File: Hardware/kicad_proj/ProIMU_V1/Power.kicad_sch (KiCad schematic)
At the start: 15 parts, among them IC1 MP2731GQC-0000-Z, SW1 SW_SPDT, U7 TPS54308, U8 TPS54308

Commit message: Updated Schematic and Layout
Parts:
- added C23, C25, C26, C28: 1uF, Capacitor_SMD:C_0402_1005Metric_Pad0.74x0.62mm_HandSolder, symbol Device:C_Small
- added C24, C27: 10uF, Capacitor_SMD:C_0402_1005Metric_Pad0.74x0.62mm_HandSolder, symbol Device:C_Small
- added D2: LED, LED_SMD:LED_0603_1608Metric, symbol Device:LED
- added L3: 1.0uH, Inductor_SMD:L_0805_2012Metric_Pad1.05x1.20mm_HandSolder, symbol Device:L
- added Q1: 2SC4213, Package_TO_SOT_SMD:SOT-323_SC-70, symbol Transistor_BJT:2SC4213
- added R14, R17, R19: 10K, Resistor_SMD:R_0402_1005Metric_Pad0.72x0.64mm_HandSolder, symbol Device:R_Small
- added R15, R16, R18: 1K, Resistor_SMD:R_0402_1005Metric_Pad0.72x0.64mm_HandSolder, symbol Device:R_Small
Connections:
- net +BATT is gone; now on net BATT: BAT1.1 (Pin_1)
- net GND: now also IC1.14 (PGND_4), IC1.15 (AGND), C23.2, C24.2, C25.2, C26.2, C27.2, Q1.2 (E), R14.1; no longer BAT1.2 (Pin_2)
- net DP: now reaches IC1.1 (DP_1)
- net DP: now also IC1.26 (DP_2), IC1.27 (DP_3)
- net INT: now reaches IC1.10 (INT)
- net NTC: now reaches IC1.11 (NTC)
- net NTC: now also R15.2, R18.1
- net VNTC: now reaches IC1.12 (VNTC)
- net VNTC: now also R18.2
- net VREF: now reaches IC1.13 (VREF)
- net VREF: now also C24.1, R17.2, R19.2
- net SYS: now reaches IC1.16 (SYS)
- net SYS: now also C25.1, L3.1
- net BATT: now reaches IC1.17 (BATT)
- net BATT: now also C26.1
- net nCE: now reaches IC1.18 (~{CE})
- net SDA: now reaches IC1.21 (SDA)
- net DISC: now reaches IC1.22 (DISC)
- net DISC: now also Q1.3 (C), R19.1
- net ILIM: now reaches IC1.24 (ILIM)
- net ILIM: now also R14.2
- net DM: now reaches IC1.25 (DM)
- net PMID: now reaches IC1.3 (PMID)
- net PMID: now also C27.1
- net SW: now reaches IC1.4 (SW)
- net SW: now also C28.2, L3.2
- net BST: now reaches IC1.8 (BST)
- net BST: now also C28.1
- net STAT: now reaches IC1.9 (STAT)
- net STAT: now also D2.1 (K)
- net BAT_I2C_SCL renamed SCL
- net BAT_OTG renamed OTG
- net USB_PWR_IN renamed IN
- net IN: now also C23.1
- new net: Q1.1 (B), R16.2
- new net: BAT1.2 (Pin_2), R15.1
- new net: D2.2 (A), R17.1
- new net DISC_PIN: R16.1
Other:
- moved on the sheet: BAT1, C12, C13, C14, C15, IC1, L1, L2, R10, R7, R8, R9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

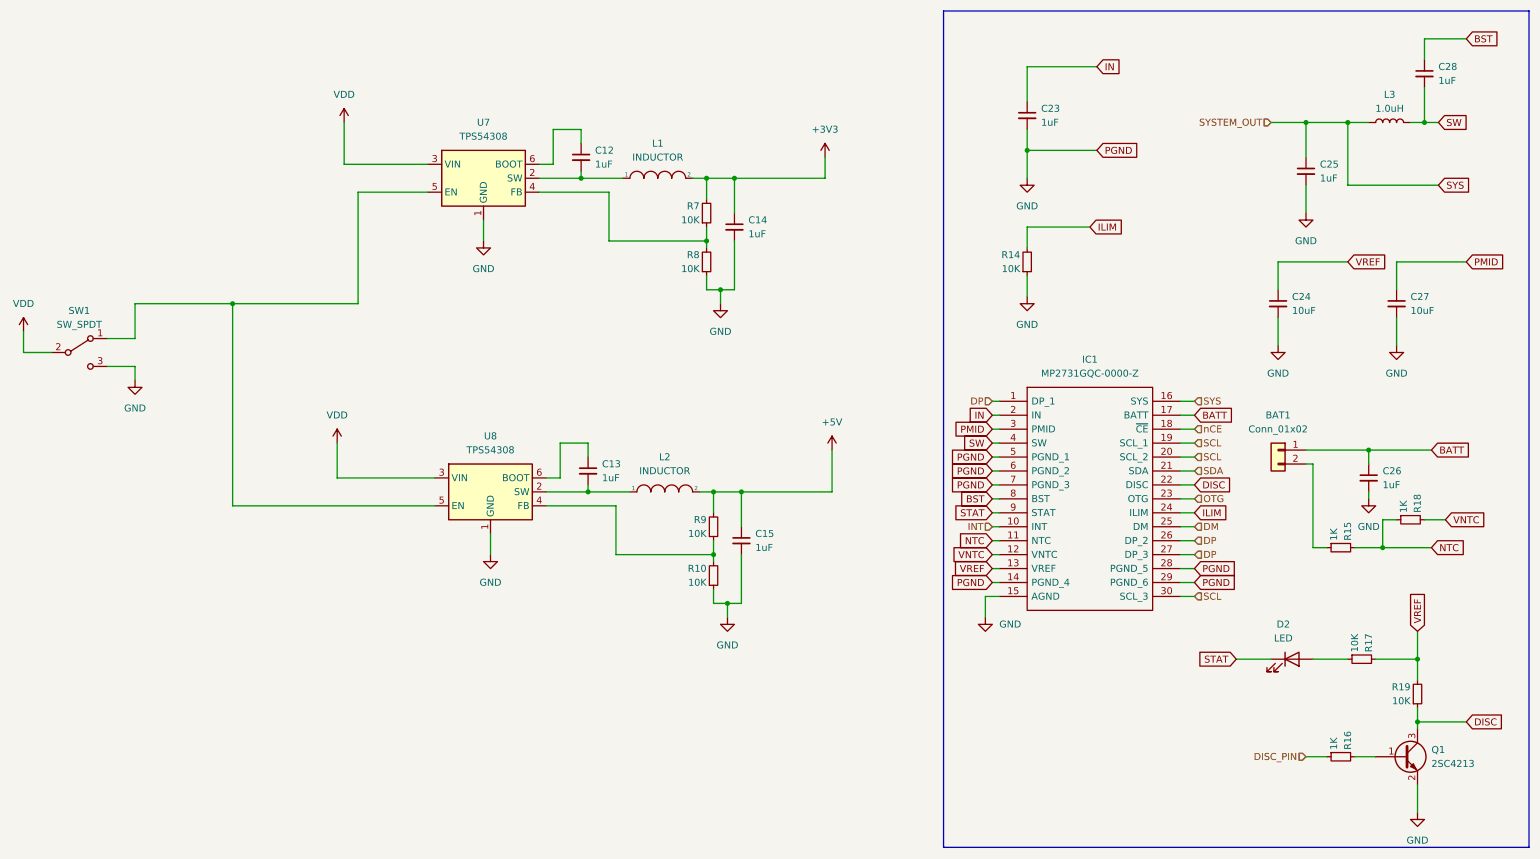
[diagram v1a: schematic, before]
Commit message: Updated Schematic
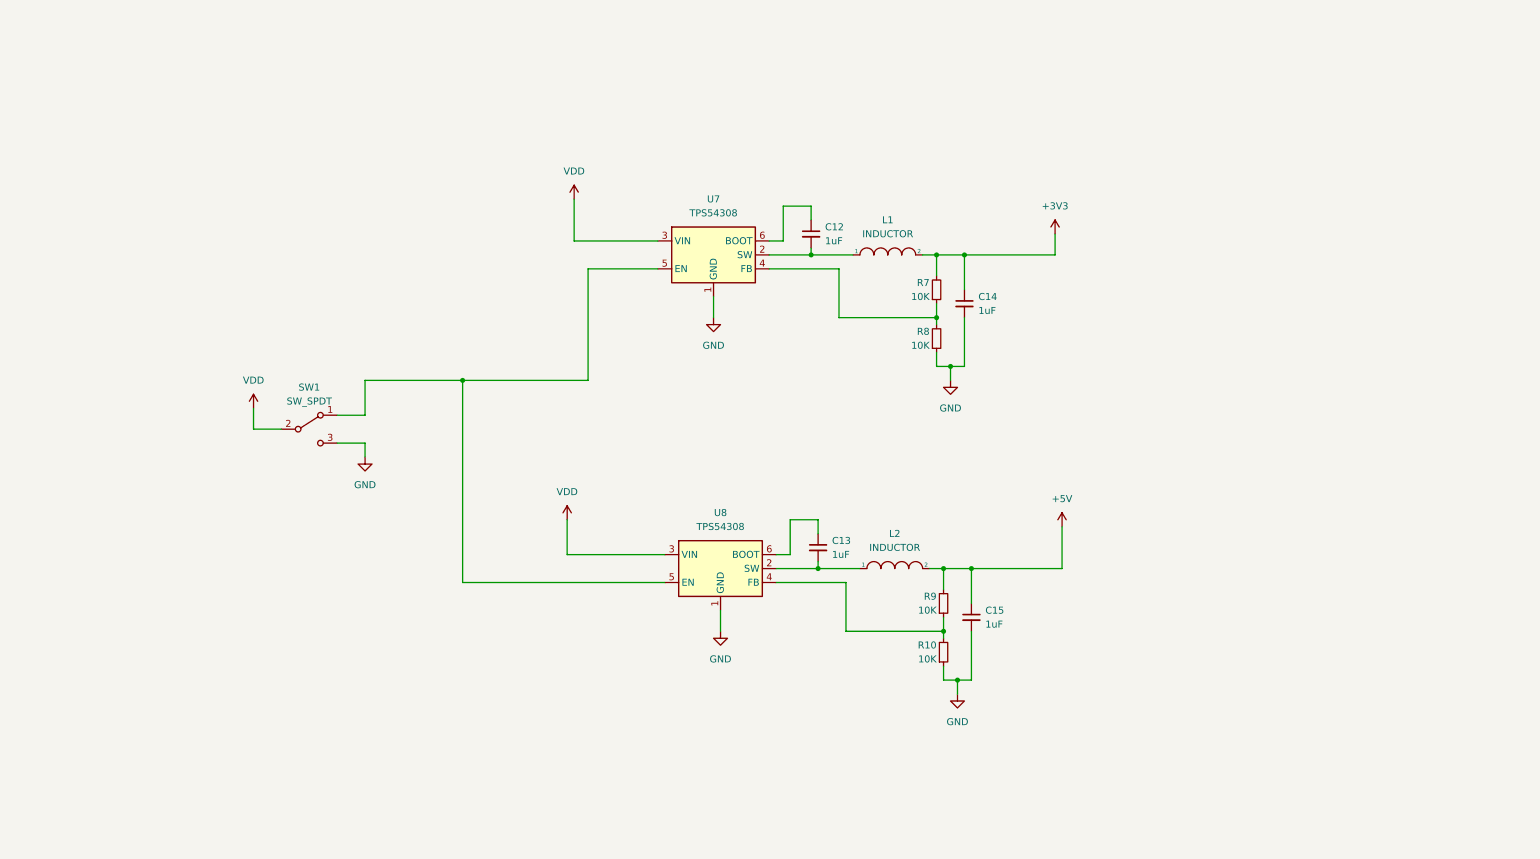
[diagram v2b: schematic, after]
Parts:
- removed BAT1: Conn_01x02, Connector_PinSocket_2.54mm:PinSocket_1x02_P2.54mm_Vertical, symbol Connector_Generic:Conn_01x02
- removed C23, C25, C26, C28: 1uF, Capacitor_SMD:C_0402_1005Metric_Pad0.74x0.62mm_HandSolder, symbol Device:C_Small
- removed C24, C27: 10uF, Capacitor_SMD:C_0402_1005Metric_Pad0.74x0.62mm_HandSolder, symbol Device:C_Small
- removed D2: LED, LED_SMD:LED_0603_1608Metric, symbol Device:LED
- removed IC1: MP2731GQC-0000-Z, footprints:MP2731GQC0000Z, symbol MP2731GQC-0000-Z:MP2731GQC-0000-Z
- removed L3: 1.0uH, Inductor_SMD:L_0805_2012Metric_Pad1.05x1.20mm_HandSolder, symbol Device:L
- removed Q1: 2SC4213, Package_TO_SOT_SMD:SOT-323_SC-70, symbol Transistor_BJT:2SC4213
- removed R14, R17, R19: 10K, Resistor_SMD:R_0402_1005Metric_Pad0.72x0.64mm_HandSolder, symbol Device:R_Small
- removed R15, R16, R18: 1K, Resistor_SMD:R_0402_1005Metric_Pad0.72x0.64mm_HandSolder, symbol Device:R_Small
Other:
- moved on the sheet: C12, C13, C14, C15, L1, L2, R10, R7, R8, R9, SW1, U7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
